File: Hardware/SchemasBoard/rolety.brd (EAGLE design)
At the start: 48.9 x 22.9 mm, 29 parts, among them IC1 LNK302, IC3 MC33269ST-3.3T3, K1 FRS1B, K2 FRS1B, T1 BC846, T2 BC846

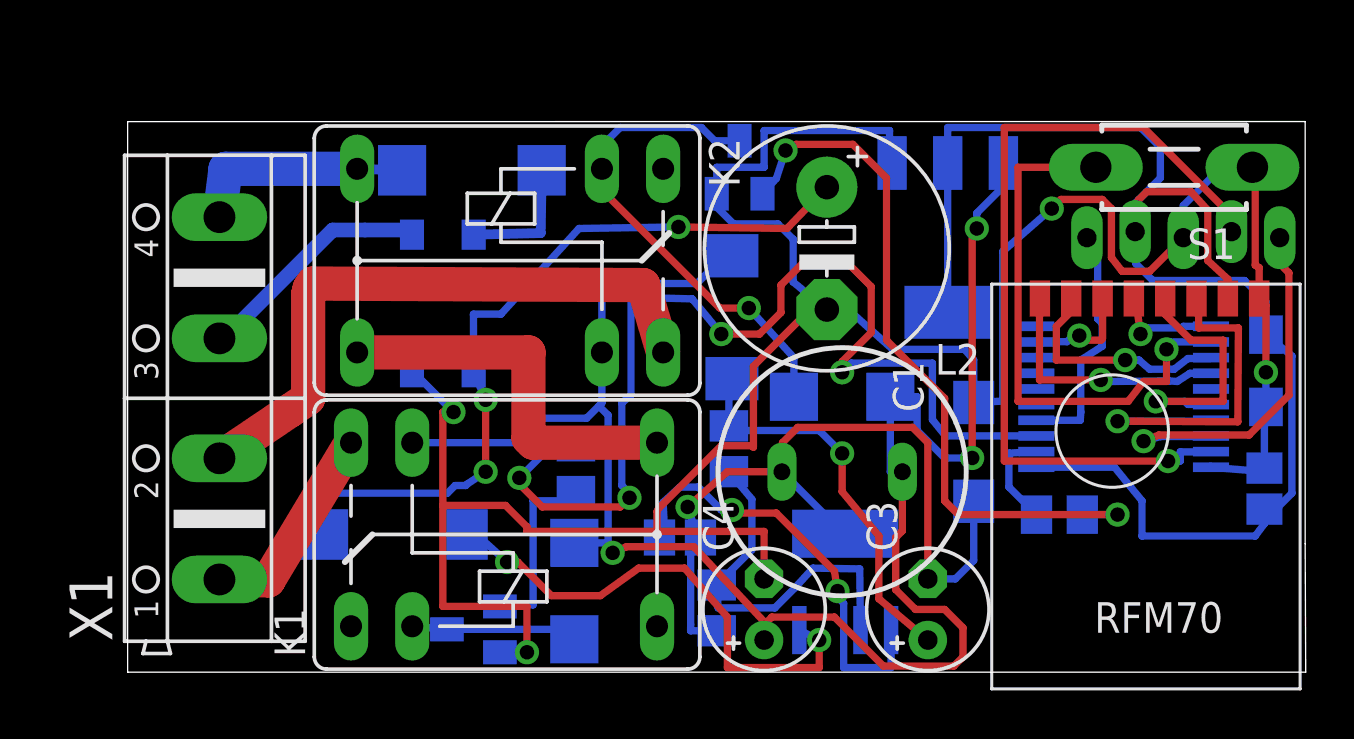
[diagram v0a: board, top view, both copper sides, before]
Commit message: aaa
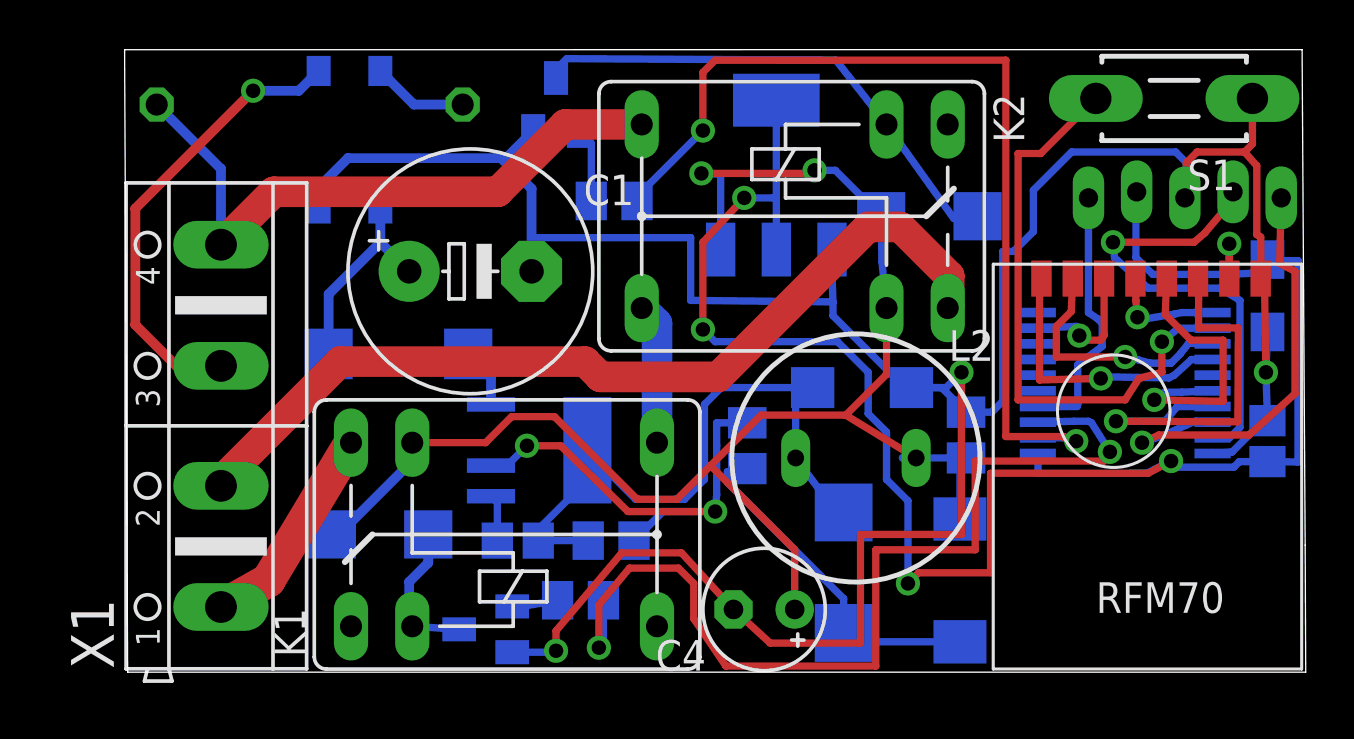
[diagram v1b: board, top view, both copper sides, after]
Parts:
- added R7: 1 K, resistor:M2012
- C3: device resistor:E2,5-5 -> resistor:SMC_C
- R2: device resistor:R2512W -> resistor:0411/12
- moved R6 22.6 mm to (19.1, 19.6), turned to 180 degrees
- moved C1 14.8 mm to (13.1, 16.6), turned to 0 degrees
- moved D4 14.5 mm to (33.4, 3.81)
- moved IC1 13.8 mm to (15.9, 9.21), turned to 90 degrees
- moved K2 12.0 mm to (30.4, 18.9)
- moved D1 8.40 mm to (9.33, 5.71), turned to 180 degrees
- moved D2 8.32 mm to (32.1, 18.9), turned to 180 degrees
- moved T2 8.05 mm to (16.6, 23.6)
- moved B1 7.82 mm to (8.06, 22.1)
- moved IC3 7.57 mm to (25.8, 20.6), turned to 0 degrees
- moved R1 7.50 mm to (10.1, 13.2)
- moved R2 7.26 mm to (6.41, 23.6)
- moved C2 6.73 mm to (15.0, 5.46)
- moved R5 5.46 mm to (17.7, 2.98), turned to 180 degrees
- moved D3 5.35 mm to (29.3, 11.8), turned to 180 degrees
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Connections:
- net GND: now also R7.1
- net N$27: now also R7.2
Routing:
- net N$6: track 4.15 -> 39.8 mm, vias 0 -> 2
- net N$28: track 30.2 -> 3.11 mm, vias 2 -> 0
- net N$2: track 32.3 -> 8.62 mm, vias 3 -> 0
- net N$17: track 59.2 -> 79.6 mm, vias 0 -> 5
- net N$1: track 21.4 -> 2.49 mm, vias 2 -> 0
- net N$36: track 9.35 -> 26.5 mm
- net N$10: track 18.0 -> 1.95 mm, vias 2 -> 0
- net N$18: track 34.4 -> 19.2 mm
- net N$27: track 77.3 -> 64.6 mm, vias 3 -> 2
- net N$8: track 25.9 -> 37.5 mm
- net N$26: track 16.1 -> 5.85 mm
- net GND: track 113.5 -> 121.0 mm, vias 4 -> 3
- net N$4: track 13.2 -> 19.1 mm, vias 0 -> 1
- net N$15: track 7.72 -> 1.94 mm
- net N$13: track 32.7 -> 27.6 mm, vias 1 -> 0
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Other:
- board size 48.9 x 22.9 mm -> 49 x 25.8 mm

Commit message: fghf
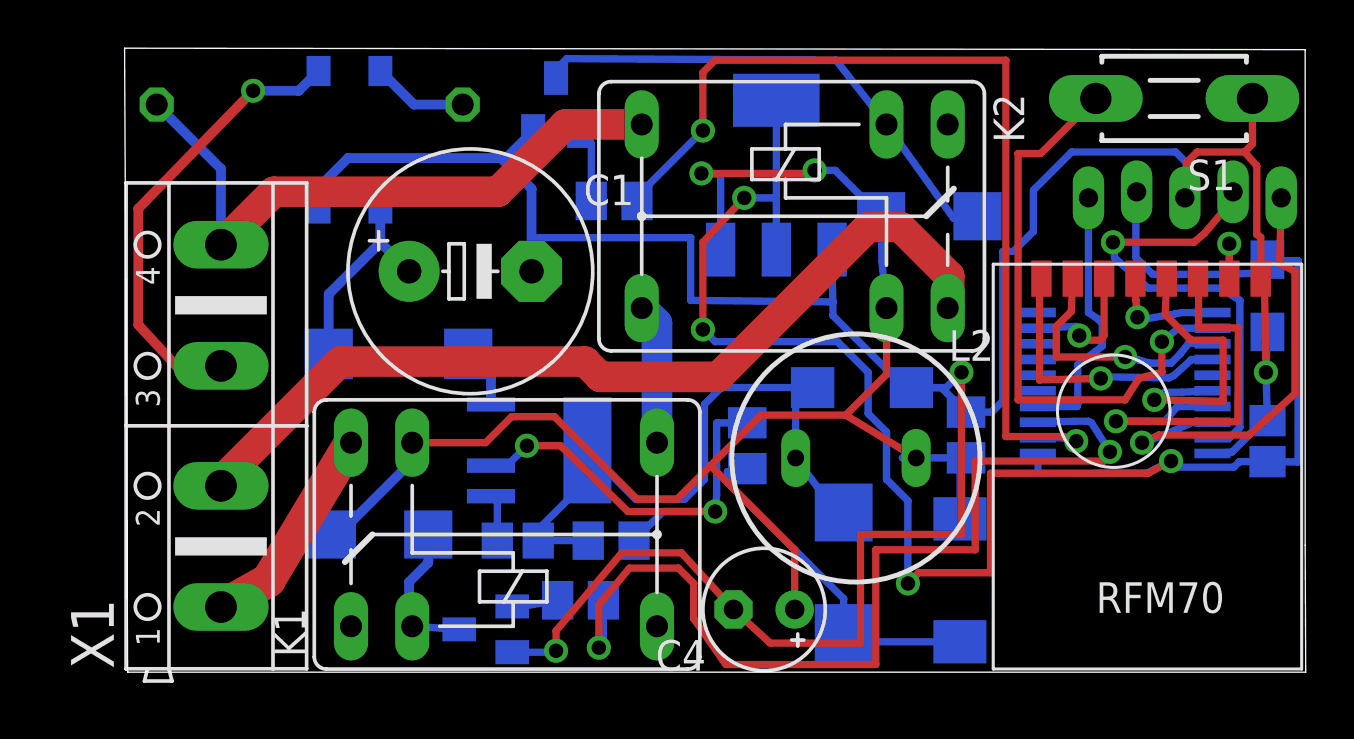
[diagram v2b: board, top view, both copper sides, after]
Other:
- board size 49 x 25.8 mm -> 49 x 25.9 mm
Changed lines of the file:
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@@
 <wire x1="-1.143" y1="0" x2="47.752" y2="0" width="0" layer="20"/>
 <wire x1="47.752" y1="0" x2="47.729" y2="5.2705" width="0" layer="20"/>
-<wire x1="47.729" y1="5.2705" x2="47.602" y2="25.838" width="0" layer="20"/>
-<wire x1="47.602" y1="25.838" x2="-1.27" y2="25.8345" width="0" layer="20"/>
-<wire x1="-1.27" y1="25.8345" x2="-1.143" y2="0" width="0" layer="20"/>
+<wire x1="47.729" y1="5.2705" x2="47.729" y2="25.838" width="0" layer="20"/>
+<wire x1="47.729" y1="25.838" x2="-1.27" y2="25.898" width="0" layer="20"/>
+<wire x1="-1.27" y1="25.898" x2="-1.143" y2="0" width="0" layer="20"/>
 </plain>
 <attributes>
@@
 <contactref element="X1" pad="3"/>
 <wire x1="2.7305" y1="12.7127" x2="0.8763" y2="12.7127" width="0.4064" layer="1"/>
-<wire x1="0.8763" y1="12.7127" x2="-0.8255" y2="14.4145" width="0.4064" layer="1"/>
-<wire x1="-0.8255" y1="14.4145" x2="-0.8255" y2="19.2405" width="0.4064" layer="1"/>
-<wire x1="-0.8255" y1="19.2405" x2="4.064" y2="24.13" width="0.4064" layer="1"/>
+<wire x1="0.8763" y1="12.7127" x2="-0.6985" y2="14.4145" width="0.4064" layer="1"/>
+<wire x1="-0.6985" y1="14.4145" x2="-0.6985" y2="19.2405" width="0.4064" layer="1"/>
+<wire x1="-0.6985" y1="19.2405" x2="4.064" y2="24.13" width="0.4064" layer="1"/>
 <via x="4.064" y="24.13" extent="1-16" drill="0.6"/>
 <wire x1="4.064" y1="24.13" x2="5.9615" y2="24.13" width="0.4064" layer="16"/>
@@
 <wire x1="21.717" y1="4.318" x2="22.352" y2="3.683" width="0.3048" layer="1"/>
 <wire x1="22.352" y1="3.683" x2="22.352" y2="2.2225" width="0.3048" layer="1"/>
-<wire x1="22.352" y1="2.2225" x2="23.6855" y2="0.254" width="0.3048" layer="1"/>
-<wire x1="23.6855" y1="0.254" x2="29.9085" y2="0.254" width="0.3048" layer="1"/>
+<wire x1="22.352" y1="2.2225" x2="23.6855" y2="0.3175" width="0.3048" layer="1"/>
+<wire x1="23.6855" y1="0.3175" x2="29.9085" y2="0.3175" width="0.3048" layer="1"/>
 <wire x1="34.036" y1="5.08" x2="34.036" y2="8.763" width="0.3048" layer="1"/>
 <wire x1="34.036" y1="8.763" x2="39.37" y2="8.763" width="0.3048" layer="1"/>
@@
 <wire x1="38.132" y1="10.414" x2="36.634" y2="10.3765" width="0.3048" layer="16"/>
 <wire x1="34.036" y1="5.08" x2="29.9085" y2="5.08" width="0.3048" layer="1"/>
-<wire x1="29.9085" y1="5.08" x2="29.9085" y2="0.254" width="0.3048" layer="1"/>
+<wire x1="29.9085" y1="5.08" x2="29.9085" y2="0.3175" width="0.3048" layer="1"/>
 </signal>
 <signal name="N$36">
